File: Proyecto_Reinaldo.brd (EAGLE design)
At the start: 60 x 40 mm, 43 parts, among them IC2 MC34063A

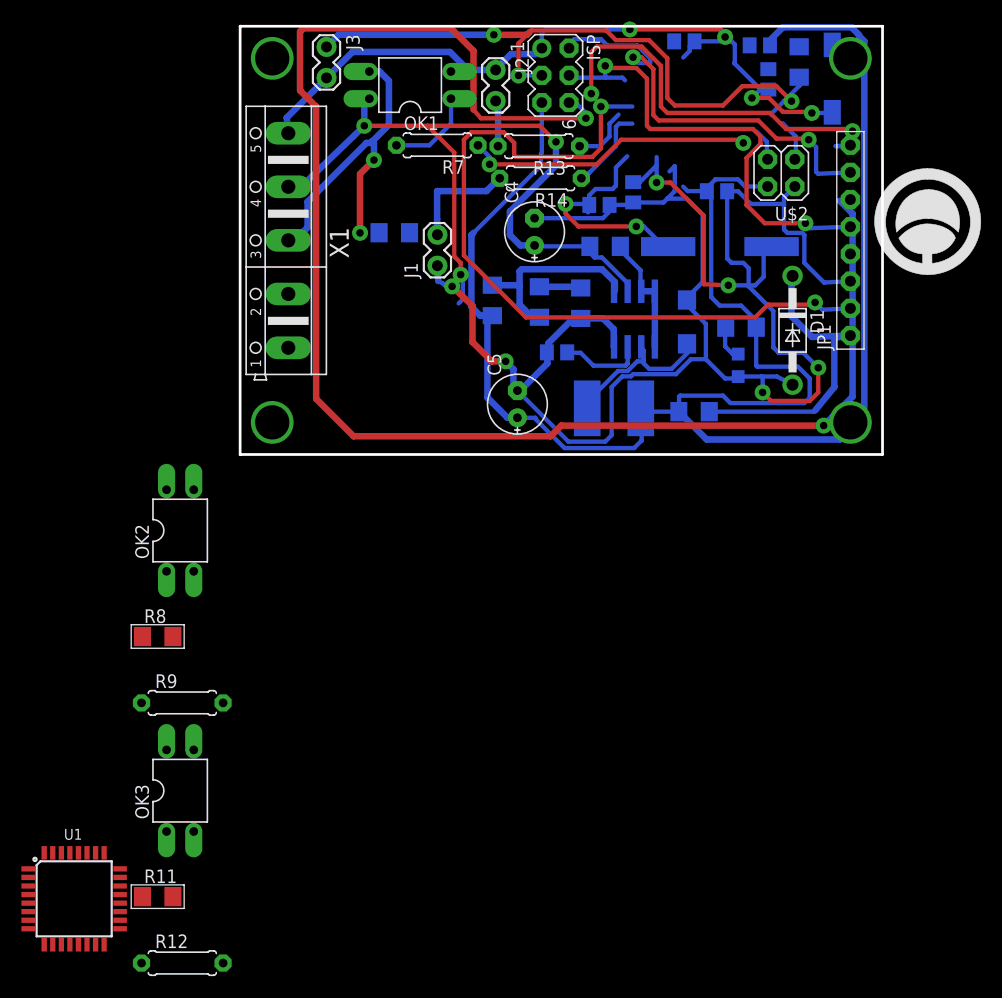
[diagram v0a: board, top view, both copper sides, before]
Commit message: Terminado posicionado componentes BRD
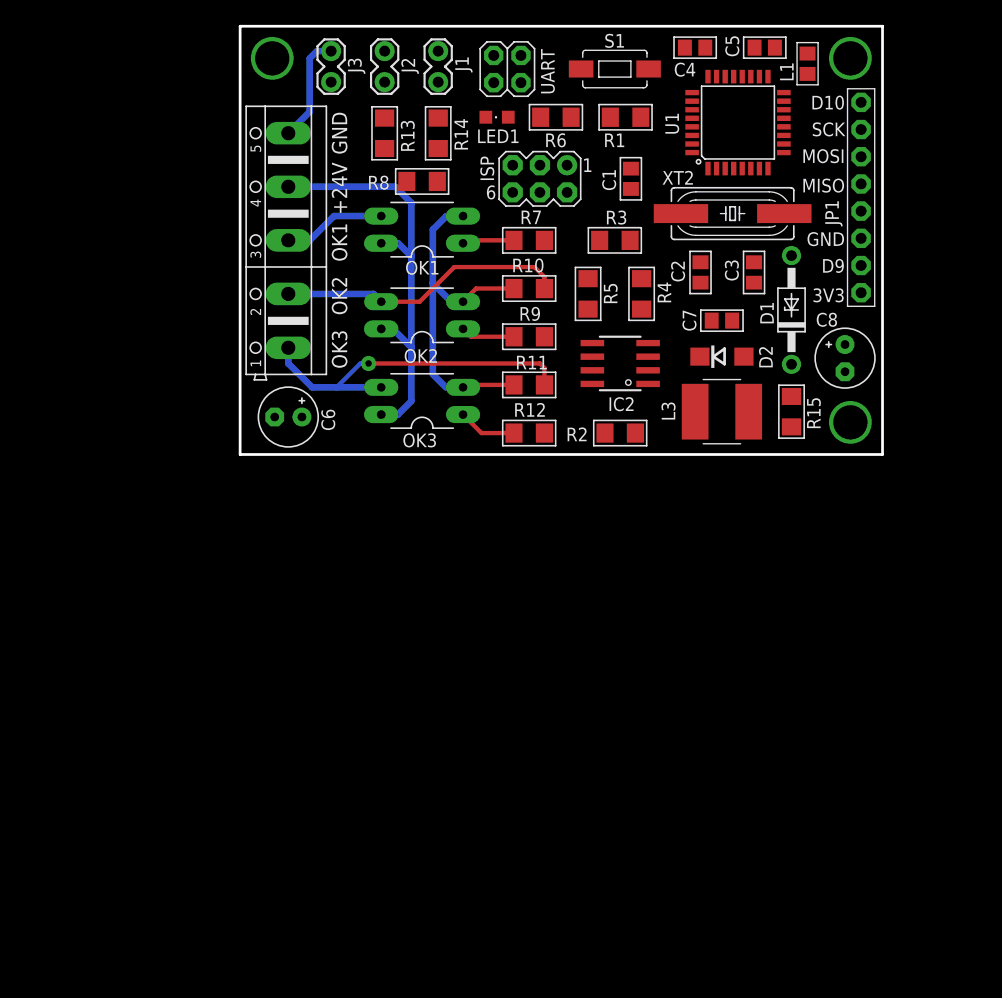
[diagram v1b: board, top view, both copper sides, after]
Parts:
- removed U$2: IPS_CIRCUITOS, isp_circuitos:ISP_CIRCUITOS
- added UART: IPS_CIRCUITOS, isp_circuitos:ISP_CIRCUITOS
- C3: value 0.1uF -> 22pF
- C4: value 22uf -> 0.1uF; device adafruit:E2,5-6E -> rcl:C0805
- C5: value 47uf -> 1uF; device adafruit:E2,5-6E -> rcl:C0805
- C6: value 22pF -> 22uf; device rcl:C0805 -> adafruit:E2,5-6E
- C8: value 1uF -> 47uf; device rcl:C0805 -> adafruit:E2,5-6E
- R1, R10, R11, R6, R8: device rcl:R1206 -> Circuitos-Creativos-RCL:R1206
- R12, R13, R14, R7, R9: value (none) -> 470R; device adafruit:0207/7 -> Circuitos-Creativos-RCL:R1206
- R2, R3, R4, R5: device resistor:R1206 -> Circuitos-Creativos-RCL:R1206
- U1: value (none) -> ATMEGA328P-AU
- moved U1 95.4 mm to (46.5, 31.0), turned to 90 degrees
- moved R12 59.2 mm to (27.0, 2.00), turned to 180 degrees
- moved R11 59.1 mm to (27.0, 6.50), turned to 180 degrees
- moved R8 49.2 mm to (17.0, 25.5)
- moved R9 47.1 mm to (27.0, 11.0), turned to 180 degrees
- moved OK3 42.8 mm to (17.0, 5.00), turned to 90 degrees
- moved C5 40.5 mm to (49.0, 38.0), turned to 180 degrees
- moved C6 35.2 mm to (4.50, 3.50), flipped to the top
- moved U$1 34.5 mm to (30.0, 17.0), flipped to the bottom
- moved LED1 32.3 mm to (24.0, 31.5), flipped to the top, turned to 90 degrees
- moved OK2 30.2 mm to (17.0, 13.0), turned to 90 degrees
- moved C8 27.0 mm to (56.5, 9.00), flipped to the top
- moved R6 26.1 mm to (29.5, 31.5), flipped to the top, turned to 180 degrees
- moved C4 22.8 mm to (42.5, 38.0), turned to 180 degrees
- moved S1 20.3 mm to (35.0, 36.0), flipped to the top, turned to 0 degrees
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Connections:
- net D5/2 renamed D5
- net D6/1 renamed D6
- net D7/4 renamed D7
- net D8/3 renamed D8
- net N$7 renamed OK3
- removed net N$3: OK2.3, R8.1, X1.2
- removed net N$6: OK1.3, R10.1, X1.3
- removed net RX1: U$2.1, U1.30
- removed net TX0: U$2.3, U1.31
- new net OK1: OK1.3, R8.1, X1.3
- new net OK2: OK2.3, R10.1, X1.2
- new net RX0: U1.30, UART.3
- new net TX1: U1.31, UART.1
- net +24V: now also C6.+; no longer C4.+
- net AREF: now also C4.1, U1.20; no longer C1.1
- net GND: now also C4.2, C5.2, C6.-, C8.-, J3.1, UART.2; no longer C4.-, C5.-, C6.2, C8.2, J3.2, U$2.2
- net N$18: now also C5.1; no longer C8.1
- net OS2: now also C3.1; no longer C6.1
- net RST: now also J3.2; no longer J3.1
- net VCC: now also C1.1, C8.+, UART.4; no longer C3.1, C5.+, U$2.4
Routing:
- net GND: track 226.3 -> 43.9 mm, vias 8 -> 0
- net VCC: track 169.6 -> 0.00 mm
- net MOSI: track 143.9 -> 0.00 mm, vias 2 -> 0
- net D9: track 72.1 -> 0.00 mm, vias 2 -> 0
- net RST: track 62.4 -> 0.00 mm, vias 3 -> 0
- net MISO: track 43.9 -> 0.00 mm, vias 2 -> 0
- net SCK: track 39.8 -> 0.00 mm, vias 2 -> 0
- net D10: track 38.5 -> 0.00 mm, vias 2 -> 0
- net OK3: track 0.00 -> 33.2 mm, vias 0 -> 1
- net +24V: track 73.3 -> 40.8 mm, vias 3 -> 0
- net N$6: track 30.7 -> 0.00 mm, vias 2 -> 0
- net +3V3: track 29.0 -> 0.00 mm
- net D2: track 27.4 -> 0.00 mm, vias 2 -> 0
- net OK2: track 0.00 -> 27.0 mm
- net OS1: track 26.4 -> 0.00 mm, vias 2 -> 0
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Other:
- board text added: "+24V"
- board text added: "3V3"
- board text added: "D10"
- board text added: "D9"
- board text added: "GND"
- board text added: "MISO"
- board text added: "MOSI"
- board text added: "OK1"
- board text added: "OK2"
- board text added: "OK3"
- board text added: "SCK"
